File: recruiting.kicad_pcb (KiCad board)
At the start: 2 copper layers, 67 x 49.5 mm, 54 parts, among them J1 Conn_01x02_Female, J2 Conn_01x02_Female, J3 Conn_01x02_Female, Q1 IRF9383M, Q2 IRF9383M, Q3 DMN2040U, U1 LM25085MM, U2 LM25085MM, U3 LM358, U4 LTC6102xMS8, U5 NE555D

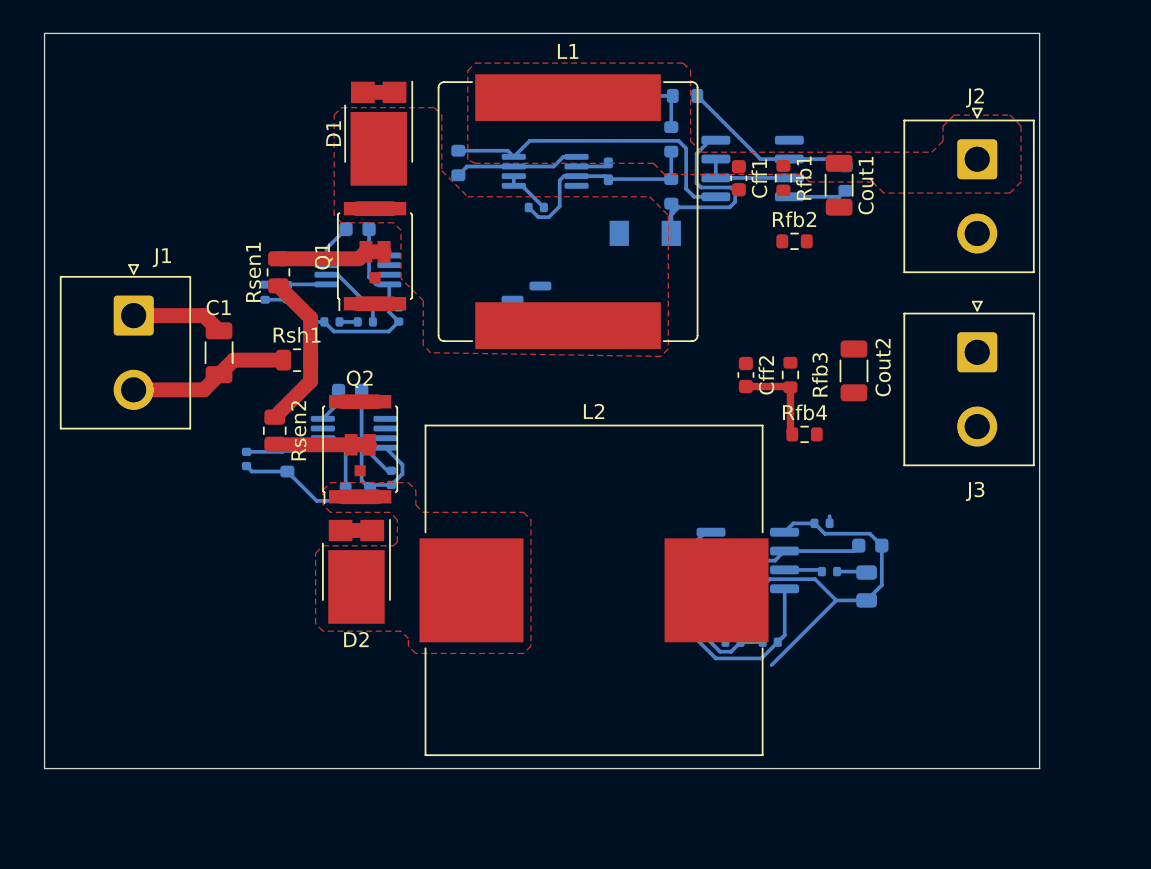
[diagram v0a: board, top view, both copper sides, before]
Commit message: ultimi dettagli al pcb
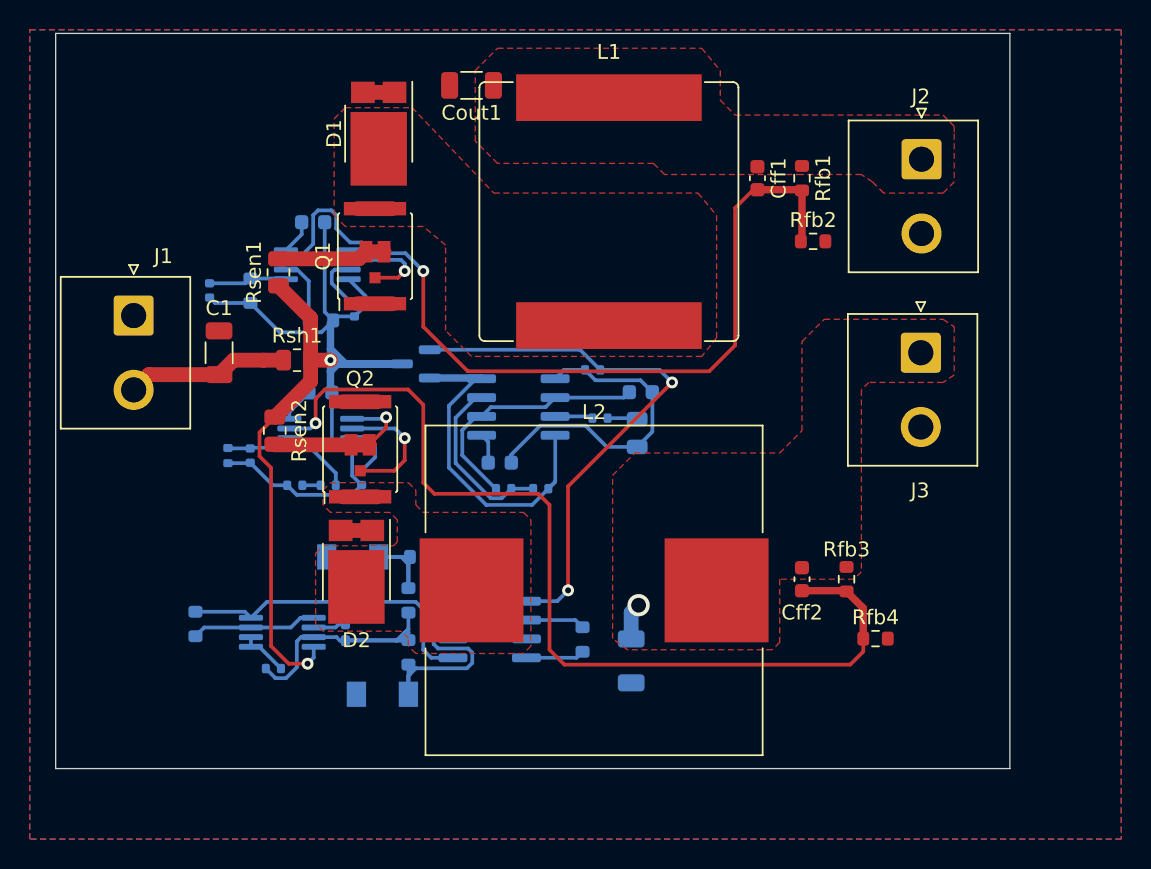
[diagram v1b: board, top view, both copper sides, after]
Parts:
- Cout2: moved to B.Cu
- moved Dz1 35.7 mm to (122.8, 99.5)
- moved R6 35.7 mm to (125.4, 90.2)
- moved R7 35.7 mm to (136.2, 95.8)
- moved Rin1 35.7 mm to (115.4, 97.8)
- moved U3 35.7 mm to (130.0, 95.1)
- moved Creg1 35.7 mm to (120.3, 95.3)
- moved Dz2 35.7 mm to (120.8, 90.2)
- moved R5 35.7 mm to (124.5, 93.2)
- moved Rout1 35.7 mm to (110.2, 94.8)
- moved U4 35.7 mm to (116.0, 95.3)
- moved R8 35.7 mm to (124.5, 96.7)
- moved Cout1 25.6 mm to (128.8, 58.5), turned to 180 degrees
- moved Cout2 24.6 mm to (139.5, 97.2)
- moved C2 18.6 mm to (140.2, 79.2)
- moved C3 18.6 mm to (130.7, 83.9)
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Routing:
- net /FB2: track 6.25 -> 65.4 mm, vias 0 -> 1
- net /FB1: track 0.00 -> 58.5 mm, vias 0 -> 1
- net /Buck controller/Vin_B: track 49.8 -> 91.7 mm, vias 0 -> 2
- net /Shunt monitor/Vout: track 0.87 -> 37.6 mm, vias 0 -> 2
- net GND: track 56.0 -> 43.6 mm
- net /GATE2: track 0.00 -> 8.60 mm, vias 0 -> 1
- net /GATE1: track 0.00 -> 6.56 mm, vias 0 -> 1
- net /Shunt monitor/Rin-: track 24.9 -> 31.4 mm
- net /ISEN2: track 7.60 -> 12.2 mm, vias 0 -> 1
- net Net-(Cvcc2-Pad2): track 0.00 -> 3.81 mm
- net Net-(Dz2-Pad1): track 4.24 -> 8.05 mm
- net Net-(Q3-Pad2): track 20.5 -> 24.0 mm
- net Net-(Cff2-Pad1): track 0.00 -> 2.48 mm, vias 0 -> 1
- added copper zone on B.Cu, net GND
- added copper zone on F.Cu, net GND
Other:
- board size 67 x 49.5 mm -> 64.2 x 49.5 mm

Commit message: ultimi dettagli al pcb
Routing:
- added copper zone on F.Cu, net Net-(Cff1-Pad1)
- added copper zone on F.Cu, net Net-(Cff2-Pad1)
- added copper zone on F.Cu, net Net-(D1-Pad3)
- added copper zone on F.Cu, net Net-(D2-Pad3)
- removed copper zone on F.Cu, net (none)
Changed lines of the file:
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@@
   (segment (start 139.5 95.775) (end 139.5 94) (width 1) (layer "B.Cu") (net 34))
   (segment (start 139.5 94) (end 140 93.5) (width 1) (layer "B.Cu") (net 34))
-  (zone (net 0) (net_name "") (layer "F.Cu") (hatch edge 0.508)
+  (zone (net 33) (net_name "Net-(Cff1-Pad1)") (layer "F.Cu") (hatch edge 0.508)
     (priority 1)
     (connect_pads (clearance 0))
@@
     )
   )
-  (zone (net 0) (net_name "") (layer "F.Cu") (hatch edge 0.508)
-    (priority 1)
+  (zone (net 13) (net_name "Net-(D1-Pad3)") (layer "F.Cu") (hatch edge 0.508)
+    (priority 3)
     (connect_pads (clearance 0))
     (min_thickness 0.254) (filled_areas_thickness no)
@@
     )
   )
-  (zone (net 0) (net_name "") (layer "F.Cu") (hatch edge 0.508)
+  (zone (net 34) (net_name "Net-(Cff2-Pad1)") (layer "F.Cu") (hatch edge 0.508)
     (priority 1)
     (connect_pads (clearance 0))
@@
     )
   )
-  (zone (net 0) (net_name "") (layer "F.Cu") (hatch edge 0.508)
+  (zone (net 14) (net_name "Net-(D2-Pad3)") (layer "F.Cu") (hatch edge 0.508)
     (priority 1)
     (connect_pads (clearance 0))
